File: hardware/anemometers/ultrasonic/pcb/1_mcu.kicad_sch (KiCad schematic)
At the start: 64 parts, among them Q1 SI2301CDS-T1-GE3, SW1 B3U-1000P, U1 TCAN330GDCNR, U2 STM32L476RGT6, U3 XC6206P332MR, X1 32.768KHz, X2 25M

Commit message: DRC clear
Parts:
- removed ?: A_A4, ProDoc_Qin-easyedapro:, symbol ProDoc_Qin-easyedapro:A_A4
- gave numbers to parts that had none: 5
- renumbered BAT to BAT1, CAN to CAN1, DEBUG to DEBUG1, I2C to I2C1, RST to RST1, SD to SD1, SPI to SPI1, SWD to SWD1, UART to UART3, USB to USB1, VBAT to VBAT1
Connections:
- net RAIN_LED: no longer names the net of U2.20 (PA4)
- no-connect marks 0 -> 8
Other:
- moved on the sheet: BAT1, C1, C10, C11, C12, C13, C14, C15, C16, C17, C18, C19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

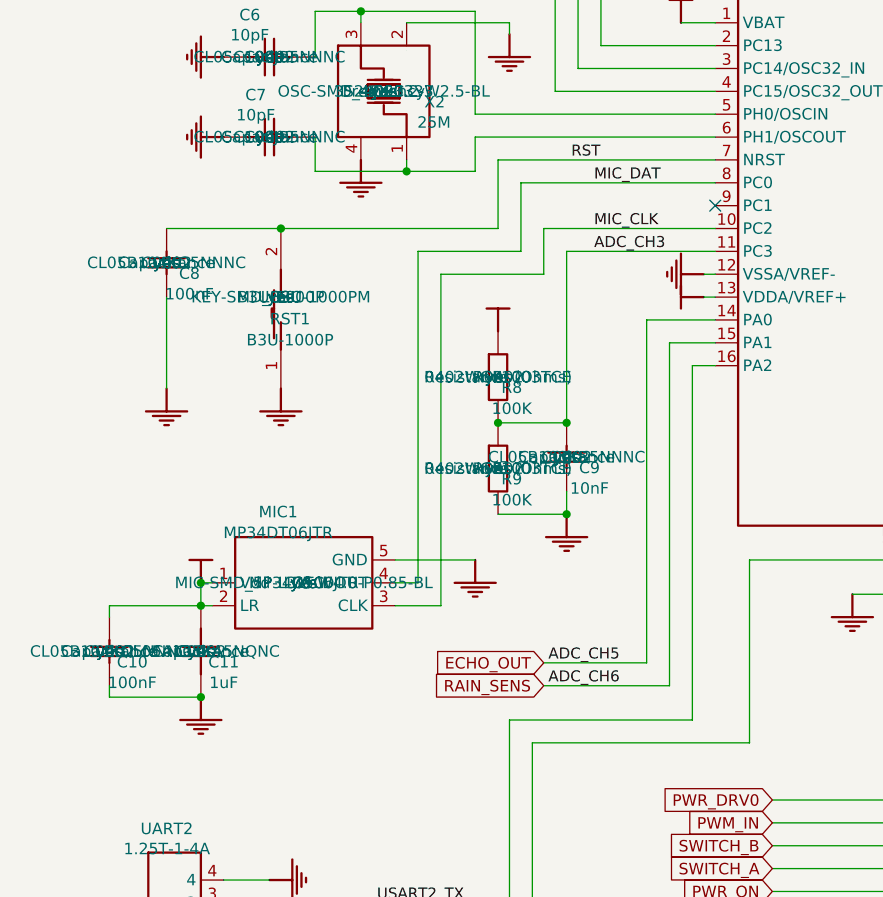
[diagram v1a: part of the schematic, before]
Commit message: update
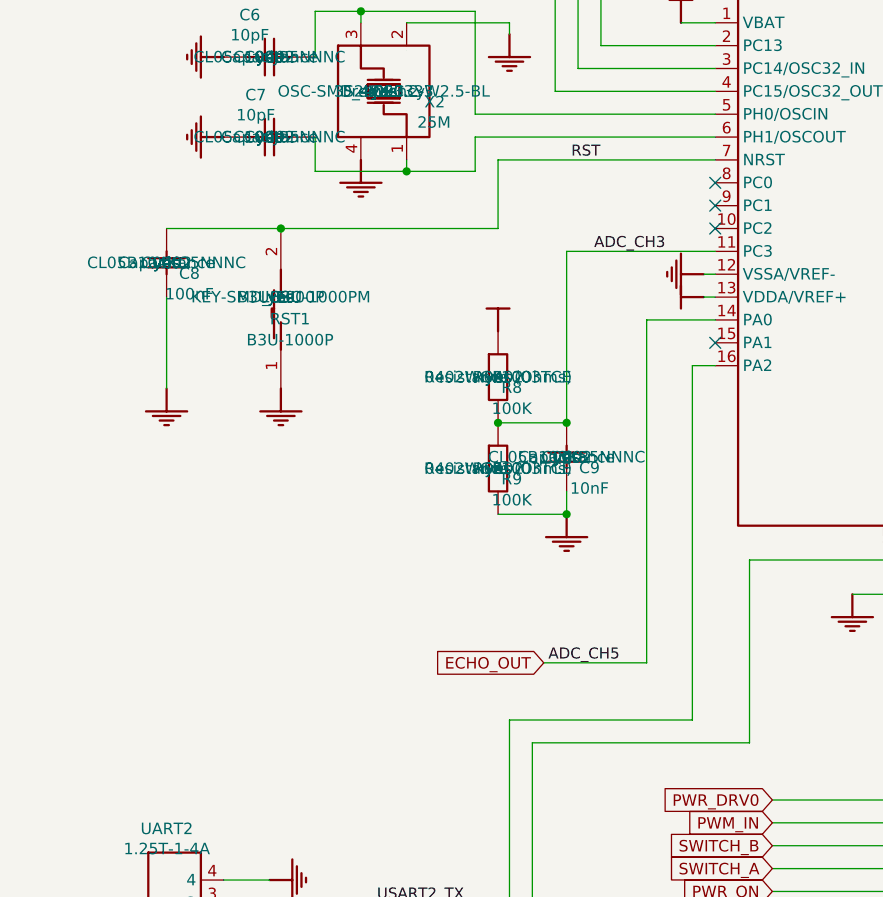
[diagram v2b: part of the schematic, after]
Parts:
- removed C10: 100nF, ProDoc_Qin-easyedapro:C0402, symbol ProDoc_Qin-easyedapro:100nF
- removed C11: 1uF, ProDoc_Qin-easyedapro:C0402, symbol ProDoc_Qin-easyedapro:1uF
- removed MIC1: MP34DT06JTR, ProDoc_Qin-easyedapro:MIC-SMD_5P-L3.0-W4.0-P0.85-BL, symbol ProDoc_Qin-easyedapro:MP34DT06JTR
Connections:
- net RAIN_SENS: no longer U2.15 (PA1)
- net MIC_CLK: no longer names the net of U2.10 (PC2)
- net MIC_DAT: no longer names the net of U2.8 (PC0)
- new net ADC_CH6: U13.
- no-connect marks 8 -> 11
